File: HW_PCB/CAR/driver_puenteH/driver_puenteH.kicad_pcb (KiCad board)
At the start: 2 copper layers, 3 parts, among them IC1 TB6612FNG, J3 Puente H, J4 Puente_H2

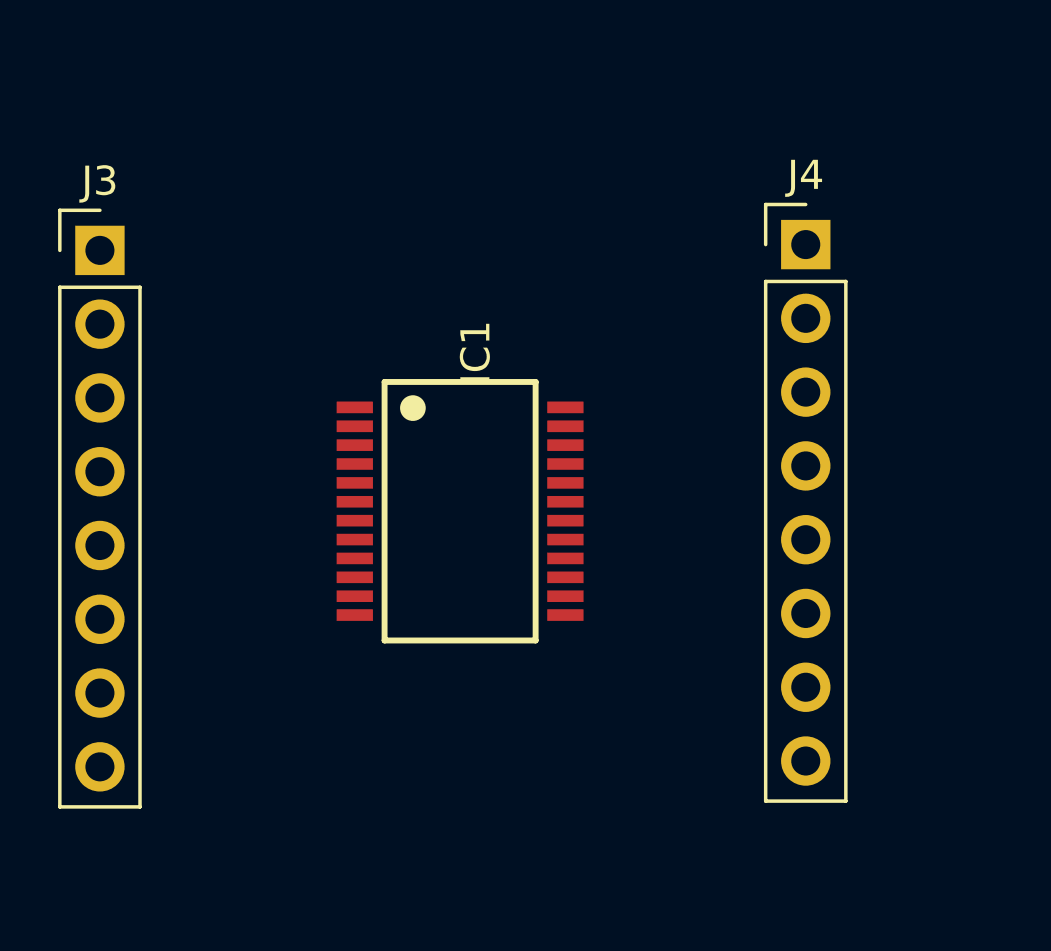
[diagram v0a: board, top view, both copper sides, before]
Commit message: Añadi nuevo proyecto del puente-H
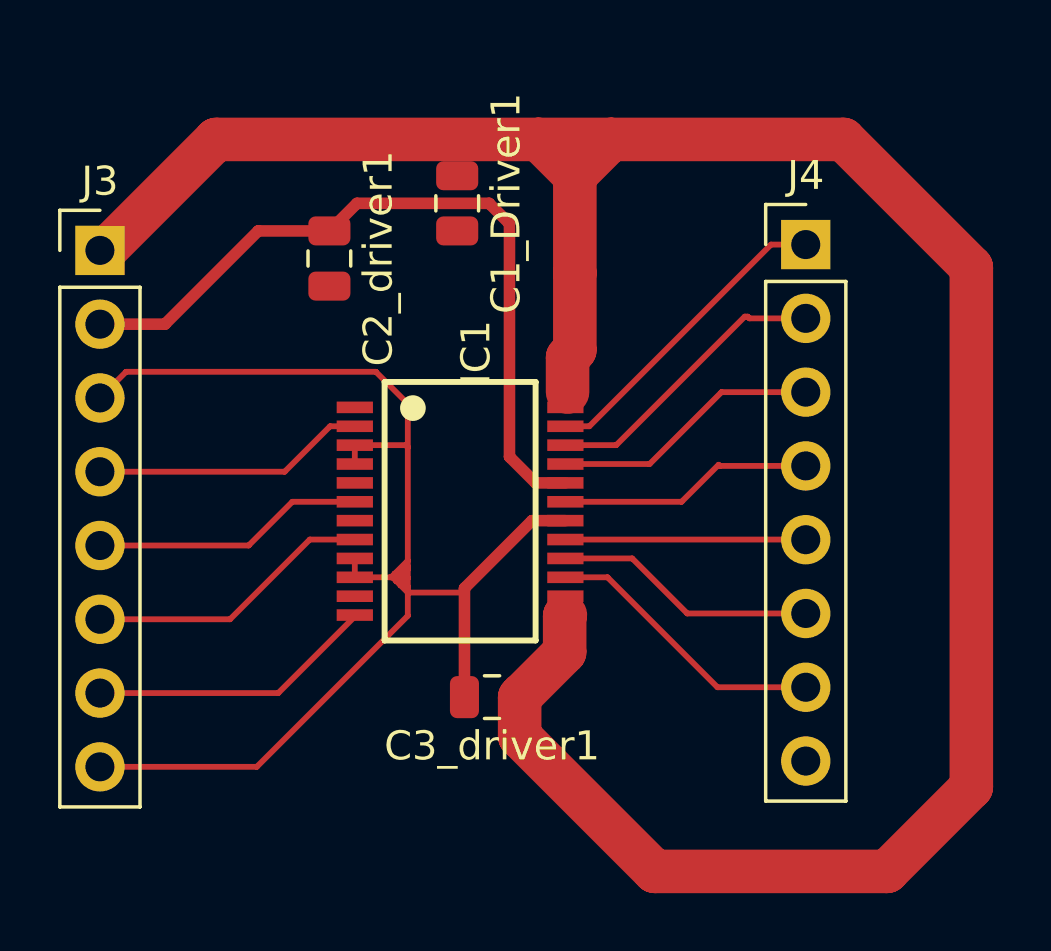
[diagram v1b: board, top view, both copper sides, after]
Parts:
- added C1_Driver1: 0.1uF, Capacitor_SMD:C_0805_2012Metric, F.Cu at (140.1, 67.9)
- added C2_driver1: 0.1uF, Capacitor_SMD:C_0805_2012Metric, F.Cu at (135.7, 69.8)
- added C3_driver1: 10uF, Capacitor_SMD:C_0805_2012Metric, F.Cu at (141.3, 84.9)
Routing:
- net /VM: track 0.00 -> 85.9 mm
- net GND: track 0.00 -> 50.3 mm
- net VCC: track 0.00 -> 26.4 mm
- net /PWMA: track 0.00 -> 10.9 mm
- net /AIN2: track 0.00 -> 10.1 mm
- net /B02: track 0.00 -> 9.92 mm
- net /B01: track 0.00 -> 9.91 mm
- net /PWMB: track 0.00 -> 9.84 mm
- net /A01: track 0.00 -> 9.42 mm
- net /A02: track 0.00 -> 9.40 mm
- net /AIN1: track 0.00 -> 9.30 mm
- net /BIN2: track 0.00 -> 9.06 mm
- net /STBY: track 0.00 -> 8.82 mm
- net /BIN1: track 0.00 -> 8.28 mm
